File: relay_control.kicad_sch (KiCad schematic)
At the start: 12 parts, among them U3 TLP3825TP1_F, U4 TLP3825TP1_F, U5 TLP3825TP1_F, U6 TLP3825TP1_F

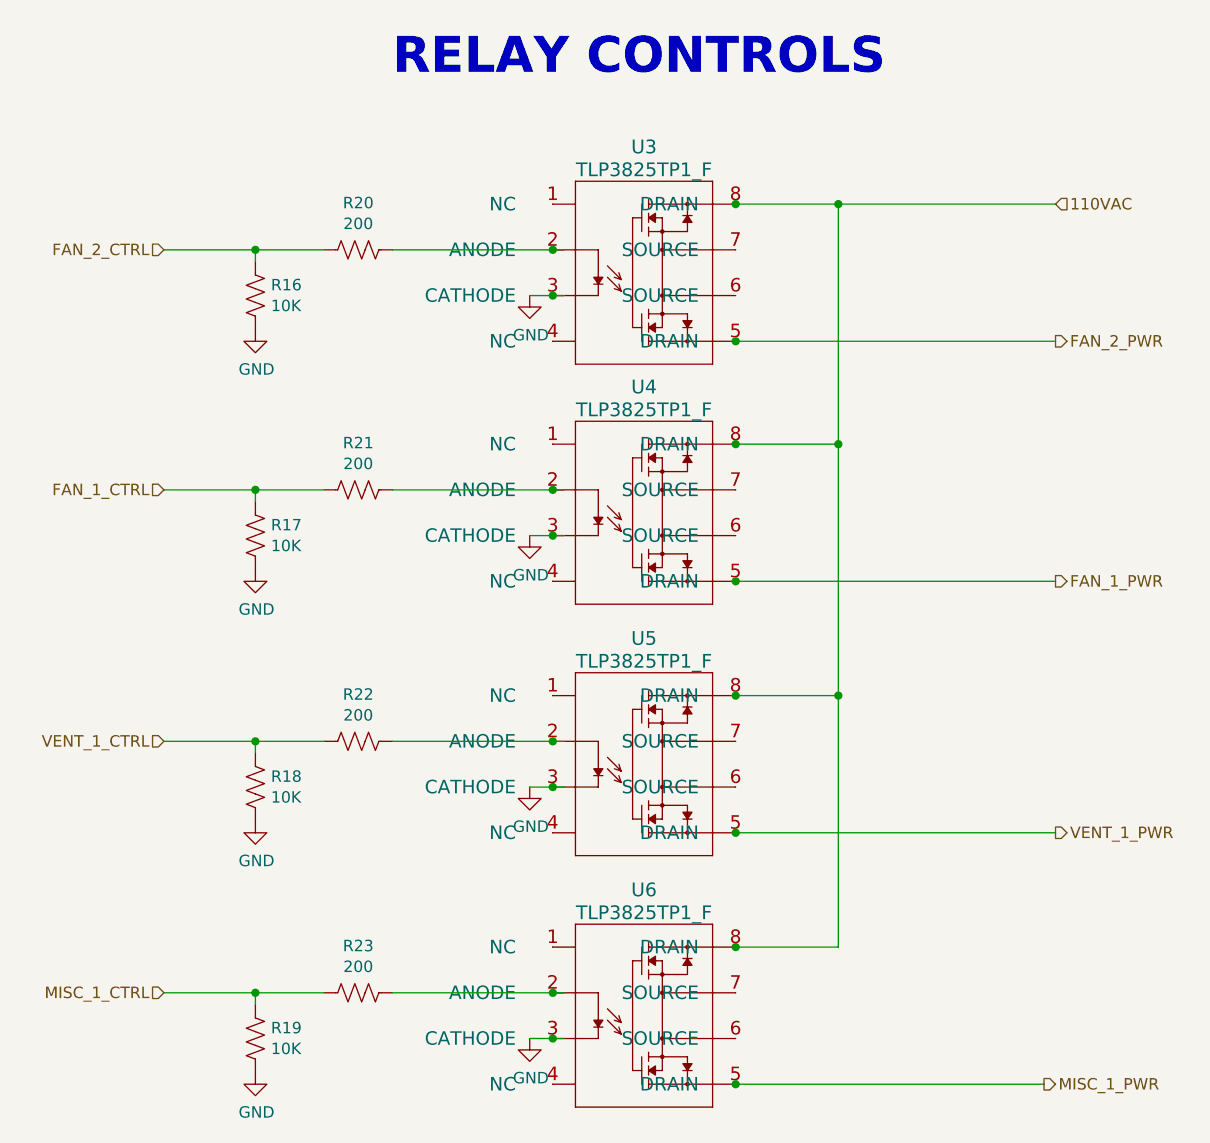
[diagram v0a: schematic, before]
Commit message: Replaced relays with smd versions.
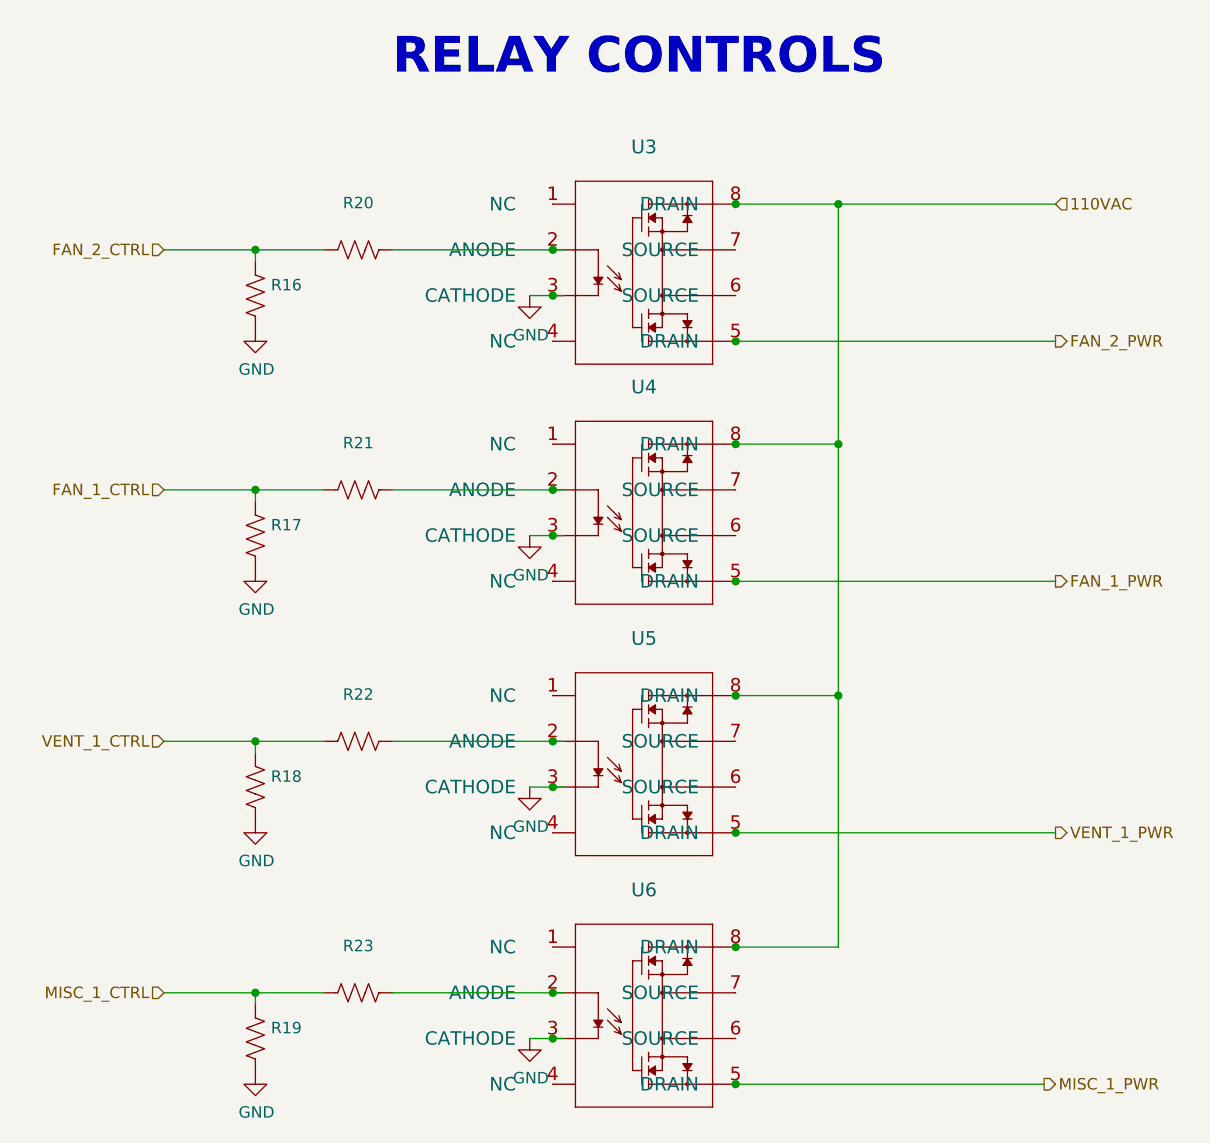
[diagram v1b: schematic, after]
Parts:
- R16, R17, R18, R19: value 10K -> (none); footprint Resistor_SMD:R_0805_2012Metric -> (none)
- R20, R21, R22, R23: value 200 -> (none); footprint Resistor_SMD:R_0805_2012Metric -> (none)
- U3, U4, U5, U6: value TLP3825TP1_F -> (none); footprint Package_DIP:DIP-8_W7.62mm -> (none)
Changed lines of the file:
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@@
     (in_bom yes) (on_board yes)
     (property "Reference" "R21" (id 0) (at 120.65 69.723 90))
-    (property "Value" "200" (id 1) (at 120.65 72.0344 90))
-    (property "Footprint" "Resistor_SMD:R_0805_2012Metric" (id 2) (at 120.396 75.946 90)
+    (property "Value" "" (id 1) (at 120.65 72.0344 90))
+    (property "Footprint" "" (id 2) (at 120.396 75.946 90)
       (effects (font (size 1.27 1.27)) hide)
     )
@@
       (effects (font (size 1.27 1.27)) (justify left))
     )
-    (property "Value" "10K" (id 1) (at 110.9472 81.153 0)
-      (effects (font (size 1.27 1.27)) (justify left))
-    )
-    (property "Footprint" "Resistor_SMD:R_0805_2012Metric" (id 2) (at 110.236 80.264 90)
+    (property "Value" "" (id 1) (at 110.9472 81.153 0)
+      (effects (font (size 1.27 1.27)) (justify left))
+    )
+    (property "Footprint" "" (id 2) (at 110.236 80.264 90)
       (effects (font (size 1.27 1.27)) hide)
     )
@@
     (in_bom yes) (on_board yes)
     (property "Reference" "R20" (id 0) (at 120.65 43.053 90))
-    (property "Value" "200" (id 1) (at 120.65 45.3644 90))
-    (property "Footprint" "Resistor_SMD:R_0805_2012Metric" (id 2) (at 120.396 49.276 90)
+    (property "Value" "" (id 1) (at 120.65 45.3644 90))
+    (property "Footprint" "" (id 2) (at 120.396 49.276 90)
       (effects (font (size 1.27 1.27)) hide)
     )
@@
       (effects (font (size 1.27 1.27)) (justify left))
     )
-    (property "Value" "10K" (id 1) (at 110.9472 54.483 0)
-      (effects (font (size 1.27 1.27)) (justify left))
-    )
-    (property "Footprint" "Resistor_SMD:R_0805_2012Metric" (id 2) (at 110.236 53.594 90)
+    (property "Value" "" (id 1) (at 110.9472 54.483 0)
+      (effects (font (size 1.27 1.27)) (justify left))
+    )
+    (property "Footprint" "" (id 2) (at 110.236 53.594 90)
       (effects (font (size 1.27 1.27)) hide)
     )
@@
     (in_bom yes) (on_board yes)
     (property "Reference" "R22" (id 0) (at 120.65 97.663 90))
-    (property "Value" "200" (id 1) (at 120.65 99.9744 90))
-    (property "Footprint" "Resistor_SMD:R_0805_2012Metric" (id 2) (at 120.396 103.886 90)
+    (property "Value" "" (id 1) (at 120.65 99.9744 90))
+    (property "Footprint" "" (id 2) (at 120.396 103.886 90)
       (effects (font (size 1.27 1.27)) hide)
     )
@@
       (effects (font (size 1.27 1.27)) (justify left))
     )
-    (property "Value" "10K" (id 1) (at 110.9472 109.093 0)
-      (effects (font (size 1.27 1.27)) (justify left))
-    )
-    (property "Footprint" "Resistor_SMD:R_0805_2012Metric" (id 2) (at 110.236 108.204 90)
+    (property "Value" "" (id 1) (at 110.9472 109.093 0)
+      (effects (font (size 1.27 1.27)) (justify left))
+    )
+    (property "Footprint" "" (id 2) (at 110.236 108.204 90)
       (effects (font (size 1.27 1.27)) hide)
     )
@@
     (in_bom yes) (on_board yes)
     (property "Reference" "R23" (id 0) (at 120.65 125.603 90))
-    (property "Value" "200" (id 1) (at 120.65 127.9144 90))
-    (property "Footprint" "Resistor_SMD:R_0805_2012Metric" (id 2) (at 120.396 131.826 90)
+    (property "Value" "" (id 1) (at 120.65 127.9144 90))
+    (property "Footprint" "" (id 2) (at 120.396 131.826 90)
       (effects (font (size 1.27 1.27)) hide)
     )
@@
       (effects (font (size 1.27 1.27)) (justify left))
     )
-    (property "Value" "10K" (id 1) (at 110.9472 137.033 0)
-      (effects (font (size 1.27 1.27)) (justify left))
-    )
-    (property "Footprint" "Resistor_SMD:R_0805_2012Metric" (id 2) (at 110.236 136.144 90)
+    (property "Value" "" (id 1) (at 110.9472 137.033 0)
+      (effects (font (size 1.27 1.27)) (justify left))
+    )
+    (property "Footprint" "" (id 2) (at 110.236 136.144 90)
       (effects (font (size 1.27 1.27)) hide)
     )
@@
       (effects (font (size 1.524 1.524)))
     )
-    (property "Value" "TLP3825TP1_F" (id 1) (at 152.4 66.04 0)
-      (effects (font (size 1.524 1.524)))
-    )
-    (property "Footprint" "Package_DIP:DIP-8_W7.62mm" (id 2) (at 144.78 67.31 0)
+    (property "Value" "" (id 1) (at 152.4 66.04 0)
+      (effects (font (size 1.524 1.524)))
+    )
+    (property "Footprint" "" (id 2) (at 144.78 67.31 0)
       (effects (font (size 1.524 1.524)) hide)
     )
@@
       (effects (font (size 1.524 1.524)))
     )
-    (property "Value" "TLP3825TP1_F" (id 1) (at 152.4 39.37 0)
-      (effects (font (size 1.524 1.524)))
-    )
-    (property "Footprint" "Package_DIP:DIP-8_W7.62mm" (id 2) (at 144.78 40.64 0)
+    (property "Value" "" (id 1) (at 152.4 39.37 0)
+      (effects (font (size 1.524 1.524)))
+    )
+    (property "Footprint" "" (id 2) (at 144.78 40.64 0)
       (effects (font (size 1.524 1.524)) hide)
     )
@@
       (effects (font (size 1.524 1.524)))
     )
-    (property "Value" "TLP3825TP1_F" (id 1) (at 152.4 121.92 0)
-      (effects (font (size 1.524 1.524)))
-    )
-    (property "Footprint" "Package_DIP:DIP-8_W7.62mm" (id 2) (at 144.78 123.19 0)
+    (property "Value" "" (id 1) (at 152.4 121.92 0)
+      (effects (font (size 1.524 1.524)))
+    )
+    (property "Footprint" "" (id 2) (at 144.78 123.19 0)
       (effects (font (size 1.524 1.524)) hide)
     )
@@
       (effects (font (size 1.524 1.524)))
     )
-    (property "Value" "TLP3825TP1_F" (id 1) (at 152.4 93.98 0)
-      (effects (font (size 1.524 1.524)))
-    )
-    (property "Footprint" "Package_DIP:DIP-8_W7.62mm" (id 2) (at 144.78 95.25 0)
-      (effects (font (size 1.524 1.524)) hide)
-    )
+    (property "Value" "" (id 1) (at 152.4 93.98 0)
+      (effects (font (size 1.524 1.524)))
+    )
+    (property "Footprint" "" (id 2) (at 144.78 95.25 0)
+      (effects (font (size 1.524 1.524)) hide)
+    )
